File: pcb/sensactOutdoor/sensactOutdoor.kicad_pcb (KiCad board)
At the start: 2 copper layers, 100 x 81 mm, 132 parts, among them J1 48V, J10 CAN, J11 EXT2, J12 OW, J13 RGB, J14 CAN, J15 PWM_OUT, J16 24V, J2 Conn_01x03, J3 Conn_01x03, J4 PROG, J5 LED CC, J7 EXT1, J8 PWM_OUT, J9 230V, K1 ALDP105W, K2 ALDP105W, K3 ALDP105W, K4 ALDP105W, K5 ALDP105W, K6 ALDP105W, M1 BxxyyS-1WR, Q1 N, Q10 BC847, Q11 BC847, Q2 N, Q3 N, Q4 N, Q5 N, Q6 BC847, Q7 BC847, Q8 BC847, Q9 BC847, SW1 TERM OFF ON, SW2 RESET, U1 ESP32-WROOM-32U, U2 A6211, U3 LM2596Board, U4 ISO1050DUB, U5 AMS1117-3.3, U6 RF, U7 RX470B, U8 EL817, U9 MAX98357_MODULE

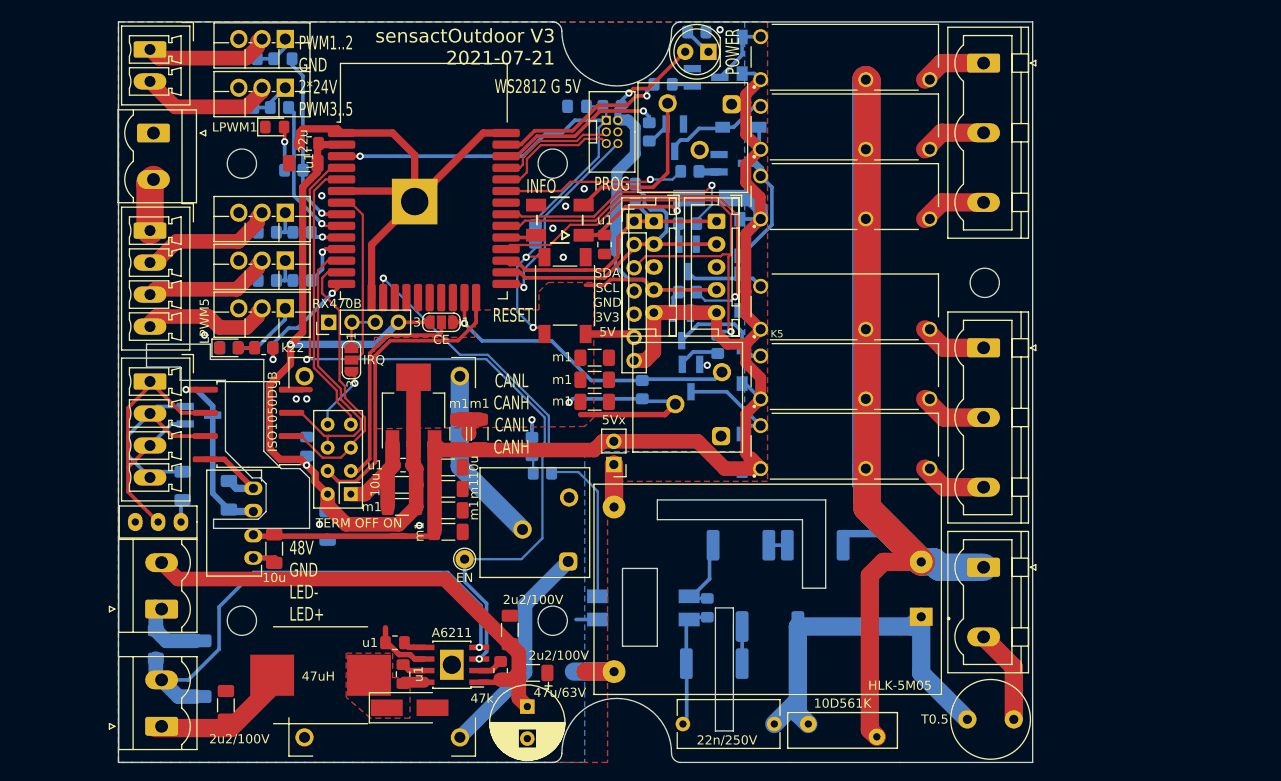
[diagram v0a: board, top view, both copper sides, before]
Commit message: Various
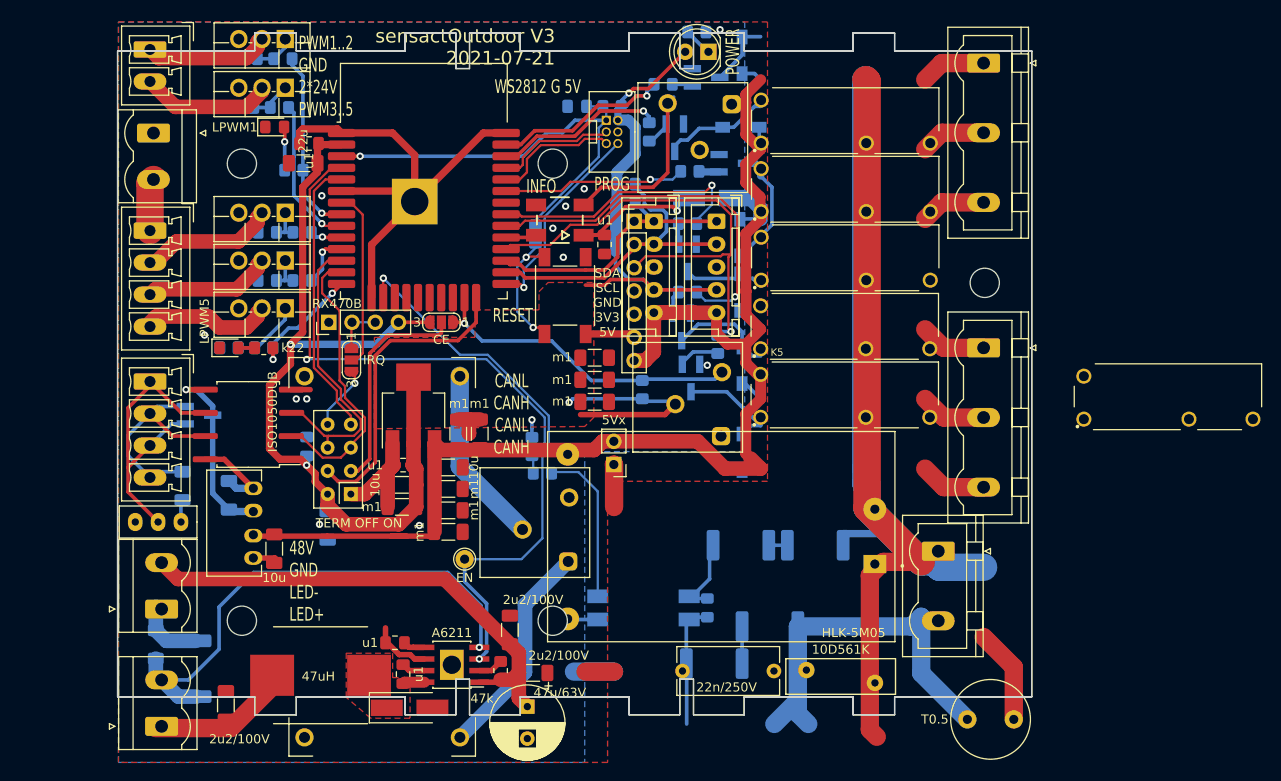
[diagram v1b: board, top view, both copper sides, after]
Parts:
- moved K6 35.8 mm to (139.8, 62.5)
- moved PS1 7.68 mm to (90.9, 77.8)
- moved K1 6.94 mm to (104.5, 32.3)
- moved K2 6.82 mm to (104.5, 39.8)
- moved K3 6.70 mm to (104.5, 47.3)
- moved RV1 5.90 mm to (100.2, 92.4)
- moved C23 5.80 mm to (96.7, 92.5)
- moved J9 5.26 mm to (114.7, 79.4)
- moved K4 2.13 mm to (104.5, 54.8)
- moved K5 2.01 mm to (104.5, 62.3)
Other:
- board size 100 x 81 mm -> 100 x 74.6 mm
- net class 230V removed
- net class 48V removed
- net class Default removed
- net class ISOLATED removed

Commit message: Various
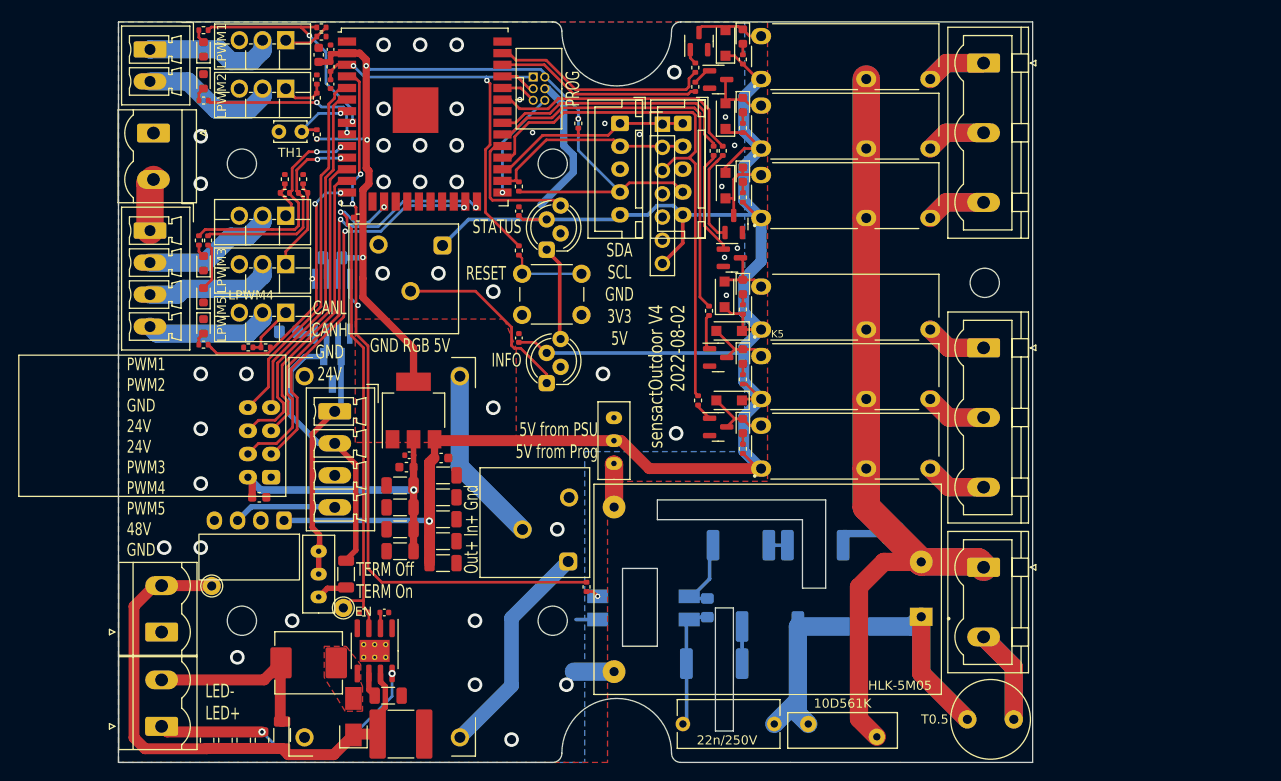
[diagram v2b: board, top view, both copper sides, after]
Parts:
- removed C25: m1, Capacitor_SMD:C_1206_3216Metric_Pad1.33x1.80mm_HandSolder
- removed C26, C27: 10u, Capacitor_SMD:C_1206_3216Metric_Pad1.33x1.80mm_HandSolder
- removed J12: OW, liebler_CONN:KF250-3.5-3P-A
- removed J14: CAN, Connector_Phoenix_MC:PhoenixContact_MCV_1,5_4-G-3.5_1x04_P3.50mm_Vertical
- removed JP1: CE, Jumper:SolderJumper-3_P1.3mm_Open_RoundedPad1.0x1.5mm_NumberLabels
- removed JP2: IRQ, Jumper:SolderJumper-3_P1.3mm_Open_RoundedPad1.0x1.5mm_NumberLabels
- removed JP3: 5Vx, Connector_PinHeader_2.54mm:PinHeader_1x02_P2.54mm_Vertical
- removed L2: 47uH, liebler_PASSIVES:L_1040
- removed M1: BxxyyS-1WR, liebler_MODULES:BxxxxS-1W
- added D16: LPWM1, LED_SMD:LED_0603_1608Metric, F.Cu at (93.3, 50.5)
- added D17: LPWM1, LED_SMD:LED_0603_1608Metric, F.Cu at (93.3, 58.1)
- added D18: LPWM1, LED_SMD:LED_0603_1608Metric, F.Cu at (93.3, 65.7)
- added D19: LPWM2, LED_SMD:LED_0603_1608Metric, F.Cu at (34.3, 28.0)
- added D20: LPWM3, LED_SMD:LED_0603_1608Metric, F.Cu at (34.3, 47.9)
- added D21: LPWM4, LED_SMD:LED_0603_1608Metric, F.Cu at (34.3, 51.4)
- added D22: NUP2105, Package_TO_SOT_SMD:SOT-23_Handsoldering, B.Cu at (48.4, 59.6)
- added D7: Betrieb, LED_THT:LED_D5.0mm-4_RGB_Staggered_Pins, F.Cu at (71.8, 46.4)
- added J6: CAN BUS, Connector_Phoenix_MC:PhoenixContact_MCV_1,5_4-G-3.5_1x04_P3.50mm_Vertical, F.Cu at (48.7, 64.1)
- added L1: 47u, Inductor_SMD:L_Abracon_ASPI-0630LR, F.Cu at (45.8, 91.6)
- added R10: 1R, Resistor_SMD:R_0805_2012Metric, F.Cu at (38.7, 100.1)
- added R34: k47, Resistor_SMD:R_0402_1005Metric, F.Cu at (93.3, 33.1)
- added R37: k47, Resistor_SMD:R_0402_1005Metric, F.Cu at (93.3, 40.7)
- added R38: k47, Resistor_SMD:R_0402_1005Metric, F.Cu at (93.3, 53.0)
- added R39: k47, Resistor_SMD:R_0402_1005Metric, F.Cu at (93.3, 60.6)
- added R40: k47, Resistor_SMD:R_0402_1005Metric, F.Cu at (93.3, 68.2)
- added R41: k22, Resistor_SMD:R_0402_1005Metric, F.Cu at (34.3, 30.1)
- added R42: k22, Resistor_SMD:R_0402_1005Metric, F.Cu at (33.8, 45.4)
- added R43: k22, Resistor_SMD:R_0402_1005Metric, F.Cu at (34.8, 45.4)
- added R44: 4k7, Resistor_SMD:R_0805_2012Metric_Pad1.20x1.40mm_HandSolder, B.Cu at (43.6, 55.4)
- added R45: K12, Resistor_SMD:R_1206_3216Metric, F.Cu at (49.9, 81.9)
- added SW3: TERM ON->, liebler_MECH:Switch_SS12D00, F.Cu at (46.9, 81.9)
- added TH1: Thermistor_NTC, Capacitor_THT:C_Disc_D3.4mm_W2.1mm_P2.50mm, F.Cu at (45.0, 33.5)
- added TP1: 48V, TestPoint:TestPoint_THTPad_D2.0mm_Drill1.0mm, F.Cu at (35.2, 83.2)
- C1: value 47u/63V -> m1; footprint Capacitor_THT:CP_Radial_D8.0mm_P3.50mm -> Capacitor_SMD:C_1206_3216Metric
- C10: value 2u2/100V -> 1n/25V; footprint Capacitor_SMD:C_1206_3216Metric_Pad1.33x1.80mm_HandSolder -> Capacitor_SMD:C_0402_1005Metric
- C11, C9: value m1 -> u1; footprint Capacitor_SMD:C_1206_3216Metric_Pad1.33x1.80mm_HandSolder -> Capacitor_SMD:C_0402_1005Metric
- C12, C14, C17: footprint Capacitor_SMD:C_1206_3216Metric_Pad1.33x1.80mm_HandSolder -> Capacitor_SMD:C_0603_1608Metric
- C13, C16: footprint Capacitor_SMD:C_0805_2012Metric_Pad1.18x1.45mm_HandSolder -> Capacitor_SMD:C_0402_1005Metric
- C15: footprint Capacitor_SMD:C_0805_2012Metric_Pad1.18x1.45mm_HandSolder -> Capacitor_SMD:C_0402_1005Metric; moved to F.Cu
- C18: value u1 -> 1u/25V; footprint Capacitor_SMD:C_0805_2012Metric_Pad1.18x1.45mm_HandSolder -> Capacitor_SMD:C_1206_3216Metric; moved to F.Cu
- C19: value m1 -> 1u/50V; footprint Capacitor_SMD:C_1206_3216Metric_Pad1.33x1.80mm_HandSolder -> Capacitor_SMD:C_1206_3216Metric
- C2, C4: value 2u2/100V -> m1; footprint Capacitor_SMD:C_1206_3216Metric_Pad1.33x1.80mm_HandSolder -> Capacitor_SMD:C_1206_3216Metric
- C20, C5, C7: footprint Capacitor_SMD:C_1206_3216Metric_Pad1.33x1.80mm_HandSolder -> Capacitor_SMD:C_1206_3216Metric
- C21: value m1 -> 10u/100V; footprint Capacitor_SMD:C_1206_3216Metric_Pad1.33x1.80mm_HandSolder -> Capacitor_SMD:C_2220_5650Metric
- C22: footprint Capacitor_SMD:C_1206_3216Metric_Pad1.33x1.80mm_HandSolder -> Capacitor_SMD:C_0603_1608Metric; moved to F.Cu
- C24: value m1 -> u1; footprint Capacitor_SMD:C_1206_3216Metric_Pad1.33x1.80mm_HandSolder -> Capacitor_SMD:C_0805_2012Metric_Pad1.18x1.45mm_HandSolder; moved to B.Cu
- C3, C6, C8: value u1 -> m1; footprint Capacitor_SMD:C_0805_2012Metric_Pad1.18x1.45mm_HandSolder -> Capacitor_SMD:C_1206_3216Metric
- D10: value 1N4148 -> SM4007PL; footprint liebler_SEMICONDUCTORS:D_SOD-123_handsolder -> Diode_SMD:D_SOD-123F; moved to F.Cu
- D11: value 1N4148 -> Stellgröße; footprint liebler_SEMICONDUCTORS:D_SOD-123_handsolder -> LED_THT:LED_D5.0mm-4_RGB_Staggered_Pins; moved to F.Cu
- D12: value 1N4148 -> SS210; footprint liebler_SEMICONDUCTORS:D_SOD-123_handsolder -> liebler_SEMICONDUCTORS:D_SMA; moved to F.Cu
- D13, D14, D15: value 1N4148 -> LPWM1; footprint liebler_SEMICONDUCTORS:D_SOD-123_handsolder -> LED_SMD:LED_0603_1608Metric; moved to F.Cu
- D2: value D -> SM4007PL; footprint Diode_SMD:D_SMA_Handsoldering -> Diode_SMD:D_SOD-123F
- D3: value POWER -> SM4007PL; footprint LED_THT:LED_D5.0mm -> Diode_SMD:D_SOD-123F
- D4: value D -> SM4007PL; footprint Diode_SMD:D_SMA_Handsoldering -> Diode_SMD:D_SOD-123F; moved to F.Cu
- D5: value INFO -> SM4007PL; footprint liebler_SEMICONDUCTORS:WS2812b_handsolder -> Diode_SMD:D_SOD-123F
- D6: value NUP2105L -> SM4007PL; footprint Package_TO_SOT_SMD:SOT-23_Handsoldering -> Diode_SMD:D_SOD-123F; moved to F.Cu
- D8, D9: footprint LED_SMD:LED_0805_2012Metric_Pad1.15x1.40mm_HandSolder -> LED_SMD:LED_0603_1608Metric
- J10: value CAN -> LED_EXT
- Q10, Q11, Q6, Q7, Q8, Q9: footprint Package_TO_SOT_SMD:SOT-23_Handsoldering -> Package_TO_SOT_SMD:SOT-23; moved to F.Cu
- R1: value 47k -> 10k; footprint Resistor_SMD:R_0805_2012Metric_Pad1.20x1.40mm_HandSolder -> Resistor_SMD:R_0402_1005Metric
- R11, R12, R14, R15, R17, R18, R19, R20, R21, R22, R23, R24, R25, R26, R29, R3, R32, R36, R5, R6, R7, R8, R9: footprint Resistor_SMD:R_0805_2012Metric_Pad1.20x1.40mm_HandSolder -> Resistor_SMD:R_0402_1005Metric; moved to F.Cu
- R13: value k22 -> 1R; footprint Resistor_SMD:R_0805_2012Metric_Pad1.20x1.40mm_HandSolder -> Resistor_SMD:R_0805_2012Metric; moved to F.Cu
- R2: value R300 -> 10k; footprint Resistor_SMD:R_1206_3216Metric_Pad1.30x1.75mm_HandSolder -> Resistor_SMD:R_0402_1005Metric; moved to F.Cu
- R27: value 4k7 -> 2R2; footprint Resistor_SMD:R_0805_2012Metric_Pad1.20x1.40mm_HandSolder -> Resistor_SMD:R_0805_2012Metric; moved to F.Cu
- R33: value 120R -> k47; footprint Resistor_SMD:R_1206_3216Metric_Pad1.30x1.75mm_HandSolder -> Resistor_SMD:R_0402_1005Metric; moved to F.Cu
- R35: footprint Resistor_SMD:R_0805_2012Metric_Pad1.20x1.40mm_HandSolder -> Resistor_SMD:R_0402_1005Metric
- R4: value Rxxx -> 1R; footprint Resistor_SMD:R_2512_6332Metric_Pad1.40x3.35mm_HandSolder -> Resistor_SMD:R_0805_2012Metric; moved to F.Cu
- SW1: value TERM OFF ON -> SW_SPDT; footprint liebler_MECH:SS12D00 -> liebler_MECH:Switch_SS12D00
- SW2: footprint liebler_MECH:SW_Push_1P1T_NO_6x6mm_H9.5mm -> Button_Switch_THT:SW_PUSH_6mm_H13mm
- U1: footprint smopla:ESP32-WROOM-32_HANDSOLDER -> RF_Module:ESP32-WROOM-32U
- U2: value A6211 -> BP1808; footprint sensact:SOIC-8_3.9x4.9mm_Pitch1.27mm_pad_handsolder -> Package_SO:SOIC-8-1EP_3.9x4.9mm_P1.27mm_EP2.41x3.3mm_ThermalVias
- U4: value ISO1050DUB -> SN65HVD230; footprint liebler_SEMICONDUCTORS:SOP-8_6.62x9.15mm_P2.54mm_handsolder -> liebler_SEMICONDUCTORS:SOIC-8_3.9x4.9mm_Pitch1.27mm_handsolder; moved to B.Cu
- U5: footprint smopla:SOT-223-3_TabPin2_HANDSOLDER -> Package_TO_SOT_SMD:SOT-223-3_TabPin2
- U6: footprint RF_Module:nRF24L01_Breakout -> liebler_MODULES:nRF24L01_Breakout
- U7: value RX470B -> DCDC_MP2315; footprint Connector_PinHeader_2.54mm:PinHeader_1x04_P2.54mm_Vertical -> liebler_MODULES:DCDC_MP2315
- moved R13 94.2 mm to (34.7, 100.1), turned to -90 degrees
- moved R33 77.0 mm to (93.3, 25.6), turned to 90 degrees
- moved D2 73.4 mm to (91.4, 31.8), turned to 90 degrees
- moved D12 67.3 mm to (50.7, 97.5), turned to 90 degrees
- moved R1 62.0 mm to (46.7, 33.8), turned to 90 degrees
- moved R27 59.6 mm to (36.7, 100.1), turned to -90 degrees
- moved D6 58.0 mm to (91.8, 62.9), turned to 180 degrees
- moved SW1 50.7 mm to (79.2, 67.3), turned to 90 degrees
- moved C3 39.1 mm to (60.5, 80.7), turned to 0 degrees
- moved K6 35.7 mm to (104.5, 67.9)
- moved J13 35.2 mm to (60.5, 46.0)
- moved D11 35.1 mm to (71.8, 61.0), turned to 90 degrees
- moved C24 31.6 mm to (48.4, 47.3)
- moved R29 31.5 mm to (51.2, 42.9), turned to 0 degrees
- moved R9 31.1 mm to (48.2, 26.4), turned to 90 degrees
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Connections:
- C1 pad 1: +48V -> +5V
- C10 pad 1: /LED_CC -> /COMP
- C11 pad 1: +3V3 -> GND
- C11 pad 2: GND -> +5V
- C15 pad 1: GND -> PROG_EN
- C15 pad 2: PROG_EN -> GND
- C18 pad 1: +3V3 -> Net-(C18-Pad1)
- C19 pad 1: +3V3 -> /LED-
- C19 pad 2: GND -> +48V
- C2 pad 1: +48V -> +3V3
- C21 pad 1: +5V -> +48V
- C24 pad 1: +3V3 -> GND
- C24 pad 2: GND -> +3V3
- C3 pad 1: GND -> +5V
- C3 pad 2: Net-(C3-Pad2) -> GND
- C4 pad 1: +48V -> +5V
- C6 pad 1: Net-(C6-Pad1) -> +3V3
- C7 pad 1: +5V -> +3V3
- C8 pad 1: /LED_SW -> +3V3
- C8 pad 2: Net-(C8-Pad2) -> GND
- C9 pad 1: +5V -> GND
- C9 pad 2: GND -> +5V
- D11 pad 1: +5V -> Net-(D11-Pad1)
- D11 pad 2: Net-(D11-Pad2) -> GND
- D12 pad 1: +5V -> +48V
- D12 pad 2: Net-(D12-Pad2) -> /SW
- D13 pad 1: +5V -> Net-(D10-Pad2)
- D14 pad 1: +5V -> Net-(D14-Pad1)
- D15 pad 1: +5V -> Net-(D15-Pad1)
- D2 pad 1: /LED_SW -> +5V
- D2 pad 2: GND -> Net-(D14-Pad1)
- D3 pad 1: Net-(D3-Pad1) -> +5V
- D3 pad 2: +3V3 -> Net-(D15-Pad1)
- D4 pad 1: Net-(C3-Pad2) -> +5V
- D4 pad 2: +5V -> Net-(D16-Pad1)
- D5 pad 1: Net-(C3-Pad2) -> +5V
- D5 pad 2: Net-(D5-Pad2) -> Net-(D17-Pad1)
- D6 pad 1: CANL -> +5V
- D6 pad 2: CANH -> Net-(D18-Pad1)
- J13 pad 2: GND -> Net-(D11-Pad1)
- J13 pad 3: Net-(D5-Pad2) -> GND
- J5 pad 1: /LED_CC -> /LED+
- J5 pad 2: /LED_CC- -> /LED-
- K2 pad A2: Net-(D11-Pad2) -> Net-(D14-Pad1)
- K3 pad A2: Net-(D12-Pad2) -> Net-(D15-Pad1)
- K4 pad A2: Net-(D13-Pad2) -> Net-(D16-Pad1)
- K5 pad A2: Net-(D14-Pad2) -> Net-(D17-Pad1)
- K6 pad A2: Net-(D15-Pad2) -> Net-(D18-Pad1)
- PS1 pad 4: Net-(JP3-Pad1) -> Net-(PS1-Pad4)
- Q10 pad 3: Net-(D14-Pad2) -> Net-(D17-Pad1)
- Q11 pad 3: Net-(D15-Pad2) -> Net-(D18-Pad1)
- Q7 pad 3: Net-(D11-Pad2) -> Net-(D14-Pad1)
- Q8 pad 3: Net-(D12-Pad2) -> Net-(D15-Pad1)
- Q9 pad 3: Net-(D13-Pad2) -> Net-(D16-Pad1)
- R1 pad 1: Net-(R1-Pad1) -> +3V3
- R1 pad 2: +48V -> THERM
- R11 pad 1: PWM5 -> CAN_TX
- R13 pad 1: Net-(D3-Pad1) -> /LED+
- R13 pad 2: GND -> +48V
- R2 pad 1: /LED_CC- -> LED_CC_EN
- R27 pad 1: +3V3 -> /LED+
- R27 pad 2: OneWire -> +48V
- R29 pad 1: MAINS -> CAN_RX
- R32 pad 2: MAINS -> CAN_RX
- R33 pad 1: CANH -> +5V
- R33 pad 2: Net-(R33-Pad2) -> Net-(D13-Pad2)
- R35 pad 1: PWM5 -> CAN_TX
- R4 pad 1: /LED_CC- -> /LED+
- R4 pad 2: GND -> +48V
- SW1 pad 1: Net-(R33-Pad2) -> Net-(PS1-Pad4)
- SW1 pad 2: CANL -> +5V
- SW1 pad 3: Net-(SW1-Pad3) -> unconnected-(SW1-Pad3)
- U1 pad 12: CANT -> MOSI
- U1 pad 13: CANR -> SCK
- U1 pad 14: PWM5 -> CAN_TX
- U1 pad 17: Net-(U1-Pad17) -> unconnected-(U1-Pad17)
- U1 pad 18: Net-(U1-Pad18) -> unconnected-(U1-Pad18)
- U1 pad 19: Net-(U1-Pad19) -> unconnected-(U1-Pad19)
- U1 pad 20: Net-(U1-Pad20) -> unconnected-(U1-Pad20)
- U1 pad 21: Net-(U1-Pad21) -> unconnected-(U1-Pad21)
- U1 pad 22: Net-(U1-Pad22) -> unconnected-(U1-Pad22)
- U1 pad 23: OneWire -> CE
- U1 pad 29: SIGNAL -> RGB_LED
- U1 pad 32: Net-(U1-Pad32) -> unconnected-(U1-Pad32)
- U1 pad 4: MAINS -> CAN_RX
- U1 pad 5: MISO -> IRQ
- U1 pad 6: GND -> MISO
- U1 pad 7: IRQ -> THERM
- U2 pad 1: +48V -> unconnected-(U2-Pad1)
- U2 pad 2: Net-(R1-Pad1) -> /COMP
- U2 pad 4: /LED_CC- -> GND
- U2 pad 5: Net-(C6-Pad1) -> /SW
- U2 pad 6: GND -> Net-(C18-Pad1)
- U2 pad 7: Net-(C8-Pad2) -> +48V
- U2 pad 8: /LED_SW -> /LED+
- U4 pad 1: +3V3 -> CAN_TX
- U4 pad 2: CANR -> GND
- U4 pad 3: CANT -> +3V3
- U4 pad 4: GND -> CAN_RX
- U4 pad 5: GND1 -> unconnected-(U4-Pad5)
- U4 pad 8: +5P -> Net-(R44-Pad1)
- U6 pad 5: CANR -> SCK
- U6 pad 6: CANT -> MOSI
- U6 pad 8: IRQ2 -> IRQ
- U7 pad 1: GND -> +5V
- U7 pad 2: IRQ1 -> GND
- U7 pad 3: IRQ1 -> +28V
- U7 pad 4: +3V3 -> unconnected-(U7-Pad4)
- U9 pad 4: Net-(U9-Pad4) -> unconnected-(U9-Pad4)
- U9 pad 5: Net-(U9-Pad5) -> unconnected-(U9-Pad5)
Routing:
- net CAN_RX: track 0.00 -> 83.3 mm, vias 0 -> 3
- net GND: track 105.4 -> 24.9 mm, vias 12 -> 44
- net +5V: track 166.8 -> 244.2 mm, vias 0 -> 1
- net MAINS: track 58.5 -> 0.00 mm, vias 1 -> 0
- net /LED_CC-: track 55.8 -> 0.00 mm, vias 1 -> 0
- net OneWire: track 35.8 -> 0.00 mm, vias 1 -> 0
- net MOSI: track 0.00 -> 34.4 mm
- net CANT: track 32.6 -> 0.00 mm
- net /LED+: track 0.00 -> 31.7 mm, vias 0 -> 2
- net CANR: track 31.5 -> 0.00 mm
- net SCK: track 0.00 -> 31.0 mm
- net CAN_TX: track 0.00 -> 29.7 mm, vias 0 -> 3
- net +3V3: track 169.1 -> 142.6 mm, vias 5 -> 6
- net Net-(D11-Pad1): track 0.00 -> 20.8 mm
- net PWM3: track 3.55 -> 24.3 mm, vias 1 -> 2
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- added copper zone on F.Cu, net /SW
- removed copper zone on F.Cu, net /LED_SW
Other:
- board size 100 x 74.6 mm -> 100 x 81 mm
- board text added: "5V from PSU 5V from Prog"
- board text added: "CANH"
- board text added: "CANL"
- board text added: "CANL CANH GND 24V"
- board text added: "GND RGB 5V"
- board text added: "INFO"
- board text added: "LED- LED+"
- board text added: "Out+ In+ Gnd"
- board text added: "PWM1 PWM2 GND 24V 24V PWM3 PWM4 PWM5 48V GND"
- board text added: "RESET"
- board text added: "STATUS"
- board text added: "TERM Off TERM On"
- board text added: "sensactOutdoor V4 2022-08-02"
- board text removed: "48V GND LED- LED+"
- board text removed: "CANL CANH CANL CANH"
- board text removed: "H"
- board text removed: "PWM1..2 GND 2*24V PWM3..5"
- board text removed: "WS2812 G 5V"
- board text removed: "sensactOutdoor V3 2021-07-21"
